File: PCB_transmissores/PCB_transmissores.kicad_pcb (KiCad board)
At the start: 2 copper layers, 147.8 x 90.2 mm, 22 parts, among them J1 Screw_Terminal_01x02

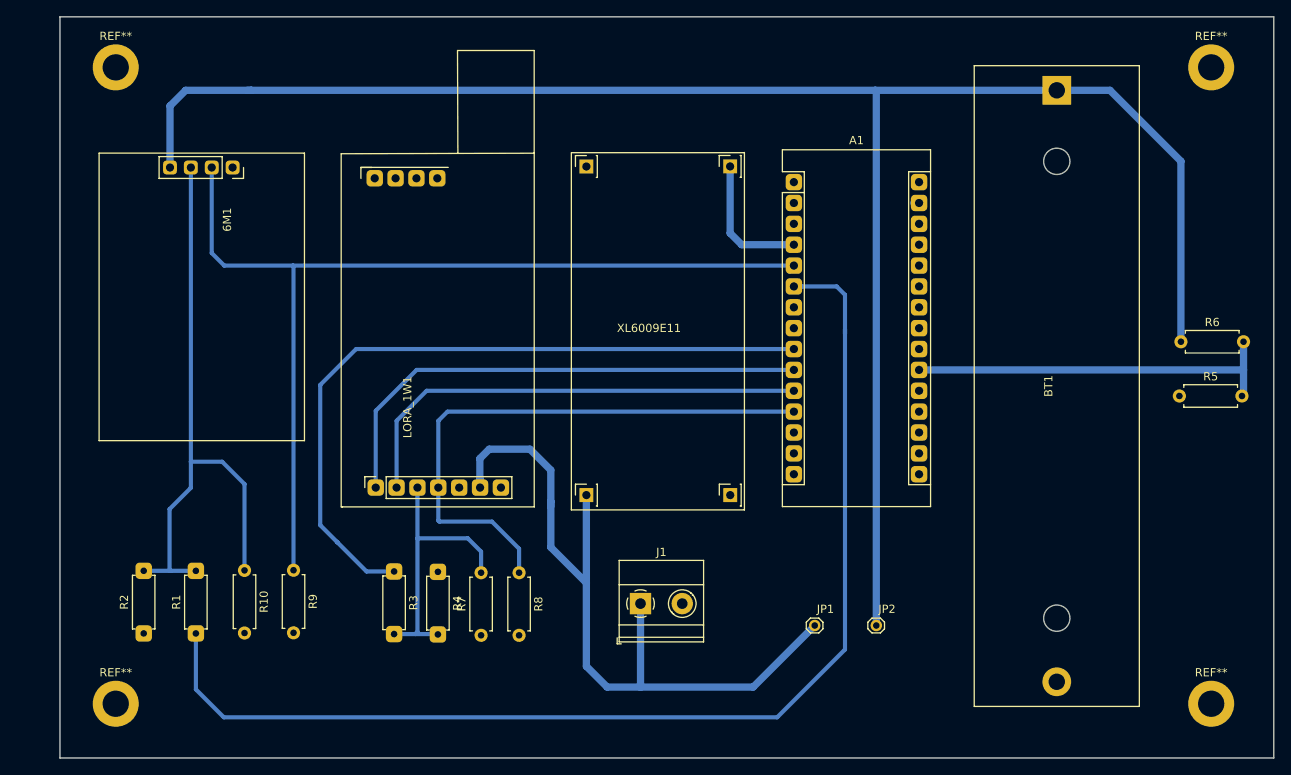
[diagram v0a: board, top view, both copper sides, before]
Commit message: atualização da placa dos transmissores
Up
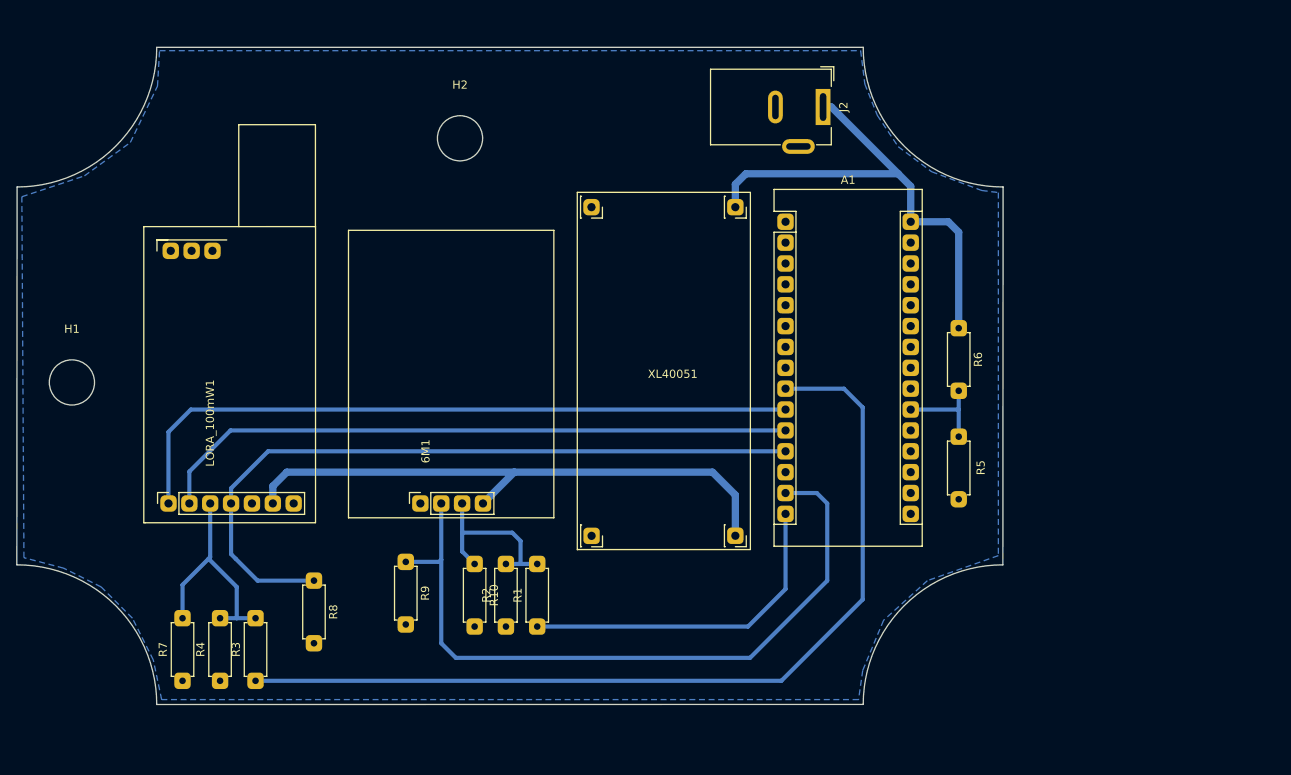
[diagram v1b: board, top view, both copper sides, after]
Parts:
- removed BT1: Battery_Cell, Battery:BatteryHolder_MPD_BH-18650-PC2
- removed J1: Screw_Terminal_01x02, TerminalBlock_Phoenix:TerminalBlock_Phoenix_MKDS-1,5-2-5.08_1x02_P5.08mm_Horizontal
- removed JP1, JP2: Jumper, TestPoint:Furo_Jumper
- removed LORA_1W1: LORA_433T30D, RF_WiFi:LORA_E32_433T30D
- removed REF** (x4): MountingHole_3.2mm_M3_DIN965_Pad, MountingHole:MountingHole_3.2mm_M3_DIN965_Pad
- removed XL6009E11: STEPUP, Converter_DCDC:STEPUP_XL6009E1
- added H1: MountingHole, MountingHole:MountingHole_5.5mm, F.Cu at (91.2, 104.4)
- added H2: MountingHole, MountingHole:MountingHole_5.5mm, F.Cu at (138.4, 74.7)
- added J2: Barrel_Jack_MountingPin, Connector_BarrelJack:BarrelJack_Wuerth_6941xx301002, F.Cu at (182.6, 70.9)
- added LORA_100mW1: LORA_433T20D, RF_WiFi:LORA_E32_433T20D, F.Cu at (104.1, 119.1)
- added XL40051: STEPDOWN, Converter_DCDC:STEPDOWN_XL4005, F.Cu at (154.4, 83.1)
- R5: value 500k -> 5k
- R6: value 5000k -> 36k
- moved 6M1 46.8 mm to (133.6, 119.1), turned to 90 degrees
- moved R2 44.1 mm to (144.0, 134.1)
- moved R1 41.6 mm to (147.8, 134.1)
- moved R7 36.8 mm to (104.6, 140.7)
- moved R5 29.7 mm to (199.1, 118.6), turned to 90 degrees
- moved R4 29.6 mm to (109.2, 140.7), turned to 90 degrees
- moved R10 28.0 mm to (140.2, 126.5)
- moved R6 27.1 mm to (199.1, 97.8), turned to 270 degrees
- moved R8 25.0 mm to (120.7, 128.5)
- moved R3 21.5 mm to (113.5, 140.7), turned to 90 degrees
- moved R9 13.7 mm to (131.8, 126.2)
- moved A1 4.93 mm to (178.1, 84.8)
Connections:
- 6M1 pad 2: D2 -> D11
- 6M1 pad 4: VIN -> 3,3v
- A1 pad 14: Net-(A1-Pad14) -> D11
- A1 pad 15: Net-(A1-Pad15) -> D12
- A1 pad 30: 7V_STEPUP -> VIN
- A1 pad 5: D2 -> Net-(A1-Pad5)
- A1 pad 6: D3 -> Net-(A1-Pad6)
- R1 pad 1: D3 -> D12
- R9 pad 1: D2 -> D11
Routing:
- net VIN: track 315.4 -> 60.2 mm
- net D3: track 143.0 -> 0.00 mm
- net D2: track 120.0 -> 0.00 mm
- net D11: track 0.00 -> 88.1 mm
- net 3,3v: track 0.00 -> 70.6 mm
- net RX_GPS: track 74.7 -> 23.2 mm
- net D12: track 0.00 -> 41.3 mm
- net A2: track 46.2 -> 11.4 mm
- net D6: track 88.0 -> 111.7 mm
- net M0: track 62.3 -> 84.9 mm
- net M1: track 58.0 -> 78.5 mm
- net D9: track 70.1 -> 88.8 mm
- net GND: track 18.4 -> 0.00 mm
- net RX_LORA: track 34.3 -> 28.3 mm
- added copper zone on B.Cu, net GND
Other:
- board size 147.8 x 90.2 mm -> 120.1 x 80 mm
